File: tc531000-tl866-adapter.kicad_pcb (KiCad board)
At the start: 2 copper layers, 43.2 x 31.5 mm, 7 parts, among them U1 TC531000, U2 27C010

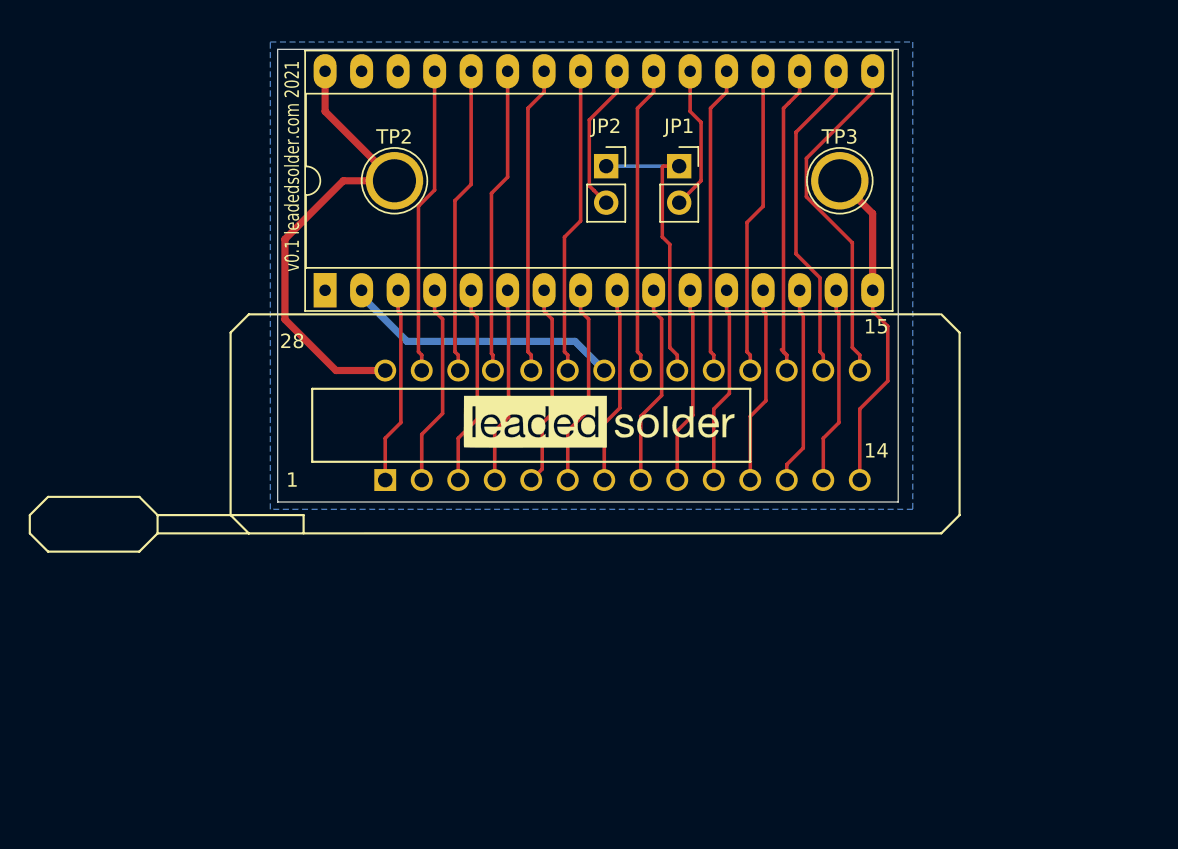
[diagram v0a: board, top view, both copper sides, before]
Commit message: V0.1 sent to osh
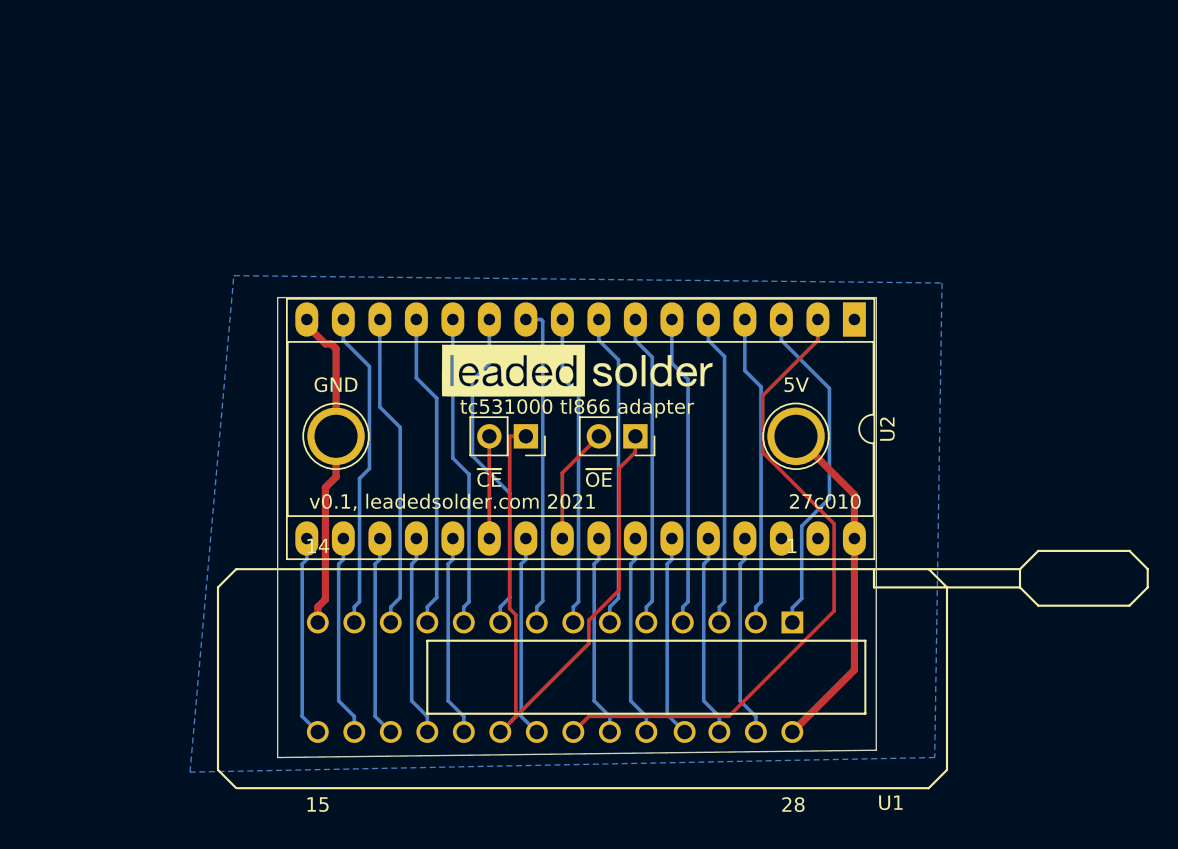
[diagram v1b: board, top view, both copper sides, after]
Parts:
- moved TP3 39.3 mm to (110.7, 52.8)
- moved U2 36.9 mm to (146.8, 44.7), turned to 270 degrees
- moved TP2 33.1 mm to (142.7, 52.8)
- moved JP1 21.6 mm to (124.0, 52.8), turned to 270 degrees
- moved JP2 18.9 mm to (131.6, 52.8), turned to 270 degrees
- moved U1 18.4 mm to (131.1, 69.6), turned to 180 degrees
- moved G*** 3.87 mm to (127.5, 48.3)
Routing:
- net /a16: track 19.4 -> 45.6 mm
- net /~TOSHIBA_CE: track 20.9 -> 45.7 mm
- net Net-(U1-Pad15): track 24.3 -> 14.0 mm
- net Net-(U1-Pad1): track 13.7 -> 23.5 mm
- net Net-(U1-Pad9): track 13.7 -> 22.9 mm
- net /5V: track 33.0 -> 24.0 mm
- net Net-(U1-Pad16): track 22.8 -> 14.0 mm
- net Net-(U1-Pad13): track 13.7 -> 22.3 mm
- net Net-(U1-Pad8): track 14.0 -> 22.4 mm
- net Net-(U1-Pad11): track 13.7 -> 21.9 mm
- net Net-(U1-Pad12): track 13.8 -> 21.9 mm
- net Net-(U1-Pad4): track 13.6 -> 21.7 mm
- net Net-(U1-Pad10): track 13.7 -> 21.7 mm
- net Net-(U1-Pad7): track 13.7 -> 21.7 mm
- net Net-(U1-Pad17): track 21.9 -> 14.0 mm
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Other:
- board size 43.2 x 31.5 mm -> 41.7 x 32 mm
- board text added: "pin 1"
- board text added: "tc531000 tl866 adapter"
- board text added: "v0.1, leadedsolder.com 2021"
- board text removed: "v0.1 leadedsolder.com 2021"
- board text removed: "vtech just kicked in, yo"
